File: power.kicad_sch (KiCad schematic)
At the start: 3 parts, among them U2 AMS1117-3.3

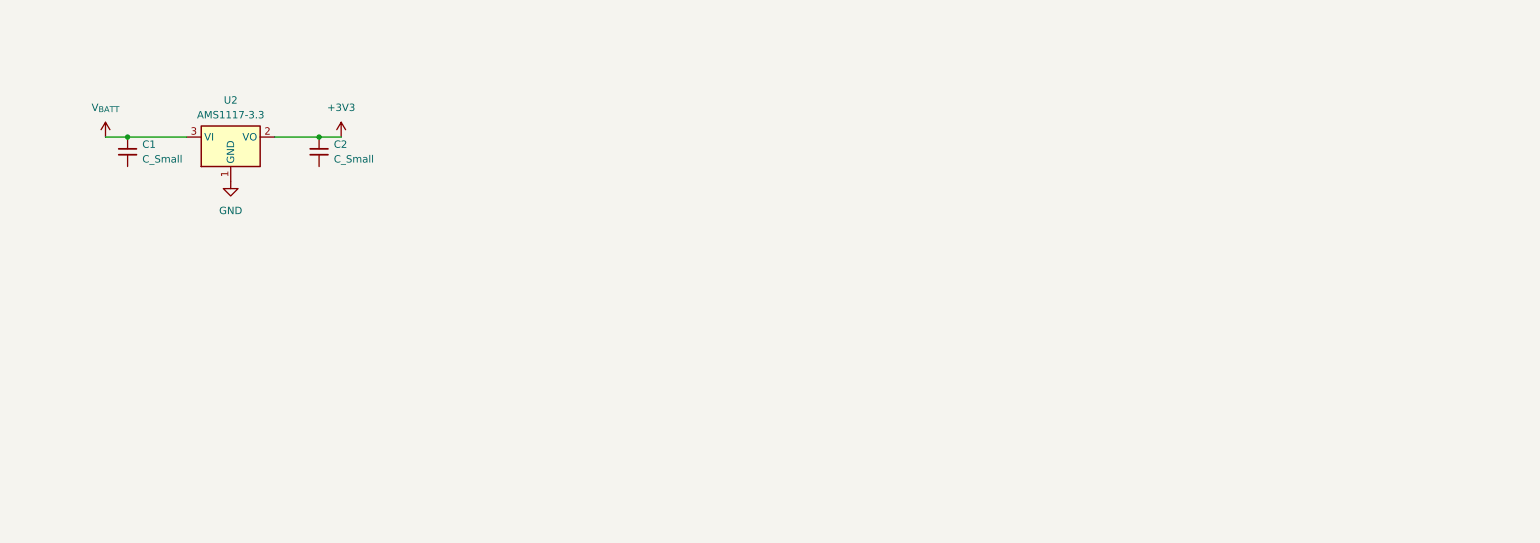
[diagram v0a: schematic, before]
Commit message: brh
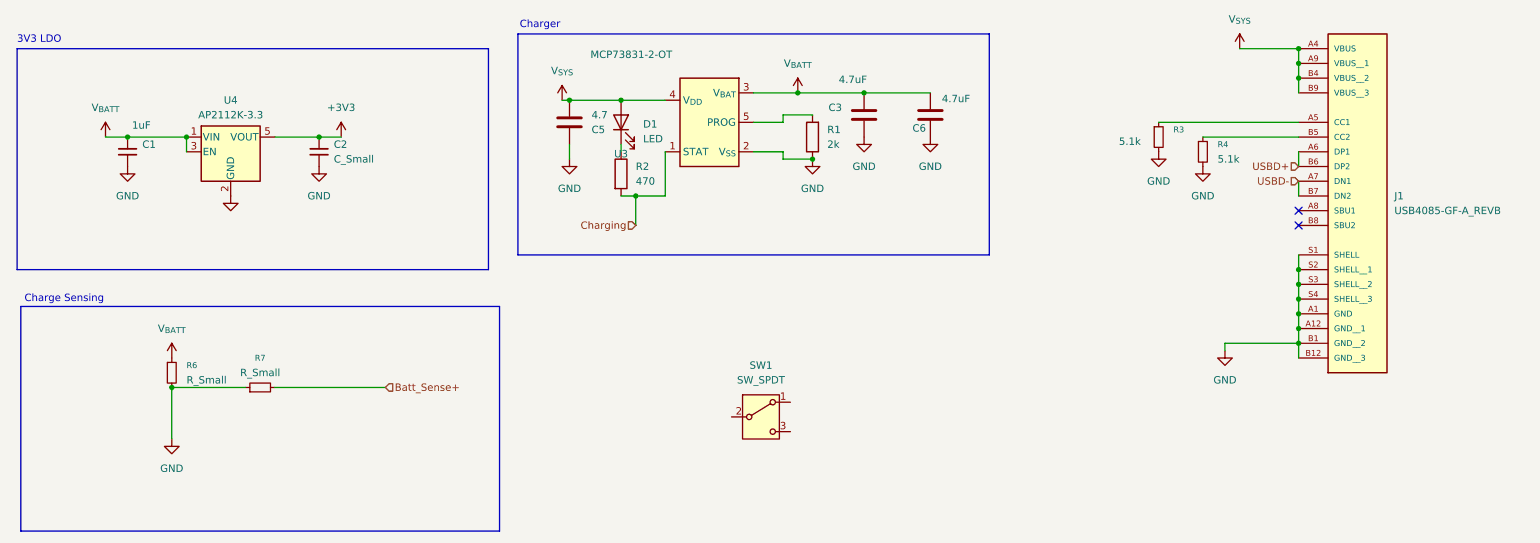
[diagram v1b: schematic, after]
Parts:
- removed U2: AMS1117-3.3, Package_TO_SOT_SMD:SOT-223-3_TabPin2, symbol Regulator_Linear:AMS1117-3.3
- added C3, C6: 4.7uF, Package_TO_SOT_SMD:SOT-23-5, symbol Device:C
- added C5: 4.7, Package_TO_SOT_SMD:SOT-23-5, symbol Device:C
- added D1: LED, symbol Device:LED
- added J1: USB4085-GF-A_REVB, USB4085-GF-A_REVB:GCT_USB4085-GF-A_REVB, symbol USB4085-GF-A_REVB:USB4085-GF-A_REVB
- added R1: 2k, symbol Device:R
- added R2: 470, symbol Device:R
- added R3, R4: 5.1k, Converter_DCDC:Converter_DCDC_RECOM_R-78B-2.0_THT, symbol Device:R_Small
- added R6, R7: R_Small, Resistor_THT:R_Array_SIP4, symbol Device:R_Small
- added SW1: SW_SPDT, Package_SO:SOIC-28W_7.5x17.9mm_P1.27mm, symbol Switch:SW_SPDT
- added U3: MCP73831-2-OT, Package_TO_SOT_SMD:SOT-23-5, symbol Battery_Management:MCP73831-2-OT
- added U4: AP2112K-3.3, Package_TO_SOT_SMD:SOT-23-5, symbol Regulator_Linear:AP2112K-3.3
- C1: value C_Small -> 1uF
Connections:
- net +3V3: now also U4.5 (VOUT)
- net GND: now also C1.2, C2.2, C3.1, C5.1, C6.1, J1.A1 (GND), J1.A12 (GND__1), J1.B1 (GND__2), J1.B12 (GND__3), J1.S1 (SHELL), J1.S2 (SHELL__1), J1.S3 (SHELL__2), J1.S4 (SHELL__3), R1.1, R3.2, R4.2, R6.2, R7.1, U3.2 (V_{SS}), U4.2 (GND)
- net V_{BATT}: now also C3.2, C6.2, R6.1, U3.3 (V_{BAT}), U4.1 (VIN), U4.3 (EN)
- new net: J1.A5 (CC1), R3.1
- new net: J1.B5 (CC2), R4.1
- new net: R1.2, U3.5 (PROG)
- new net: D1.1 (K), R2.1
- new net Batt_Sense+: R7.2
- new net Charging: R2.2, U3.1 (STAT)
- new net USBD+: J1.A6 (DP1), J1.B6 (DP2)
- new net USBD-: J1.A7 (DN1), J1.B7 (DN2)
- new net V_{SYS}: C5.2, D1.2 (A), J1.A4 (VBUS), J1.A9 (VBUS__1), J1.B4 (VBUS__2), J1.B9 (VBUS__3), U3.4 (V_{DD})
- no-connect marks 0 -> 2
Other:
- note added: "3V3 LDO"
- note added: "Charge Sensing"
- note added: "Charger"
